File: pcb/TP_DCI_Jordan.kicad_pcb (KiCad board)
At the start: 2 copper layers, 50.6 x 30 mm, 19 parts, among them J1 MICRO, J2 Display, SW1 SW_DIP_x03, U1 PCF8574

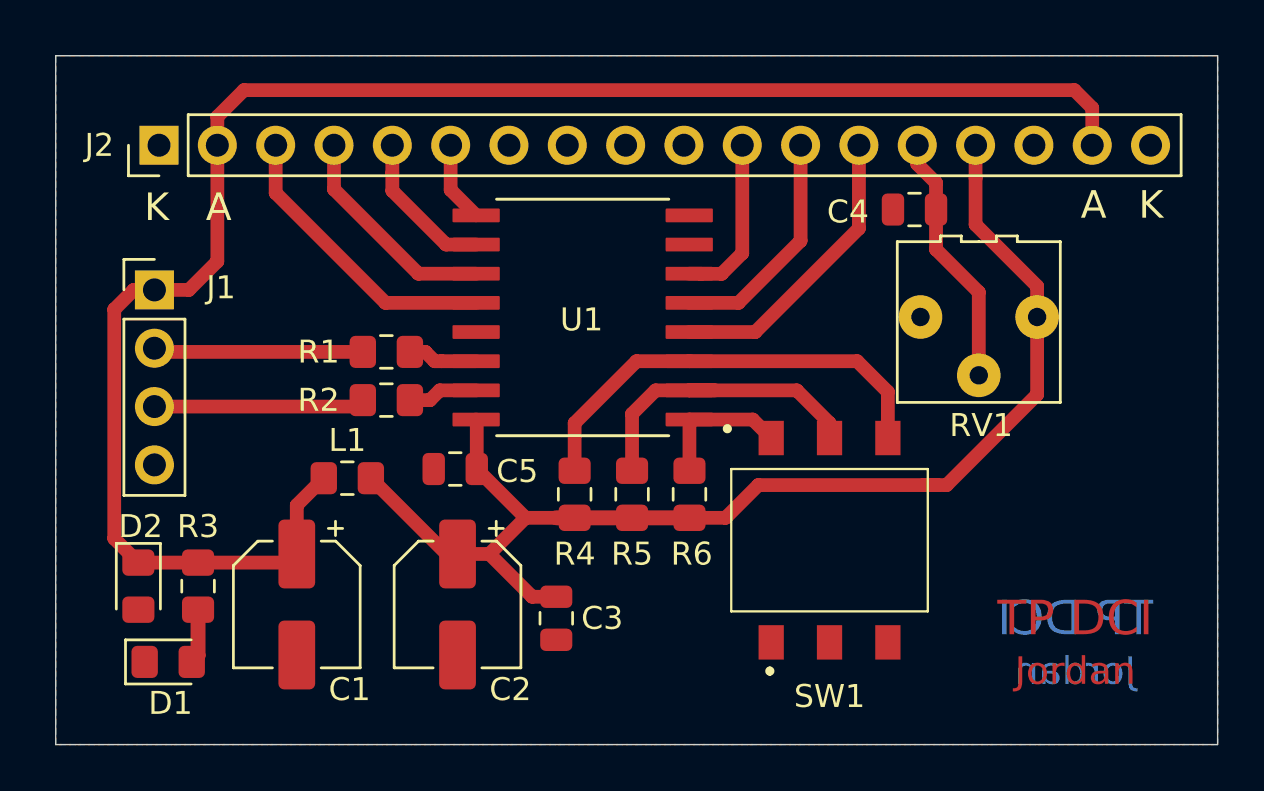
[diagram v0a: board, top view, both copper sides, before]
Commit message: medición longitudes de PCB
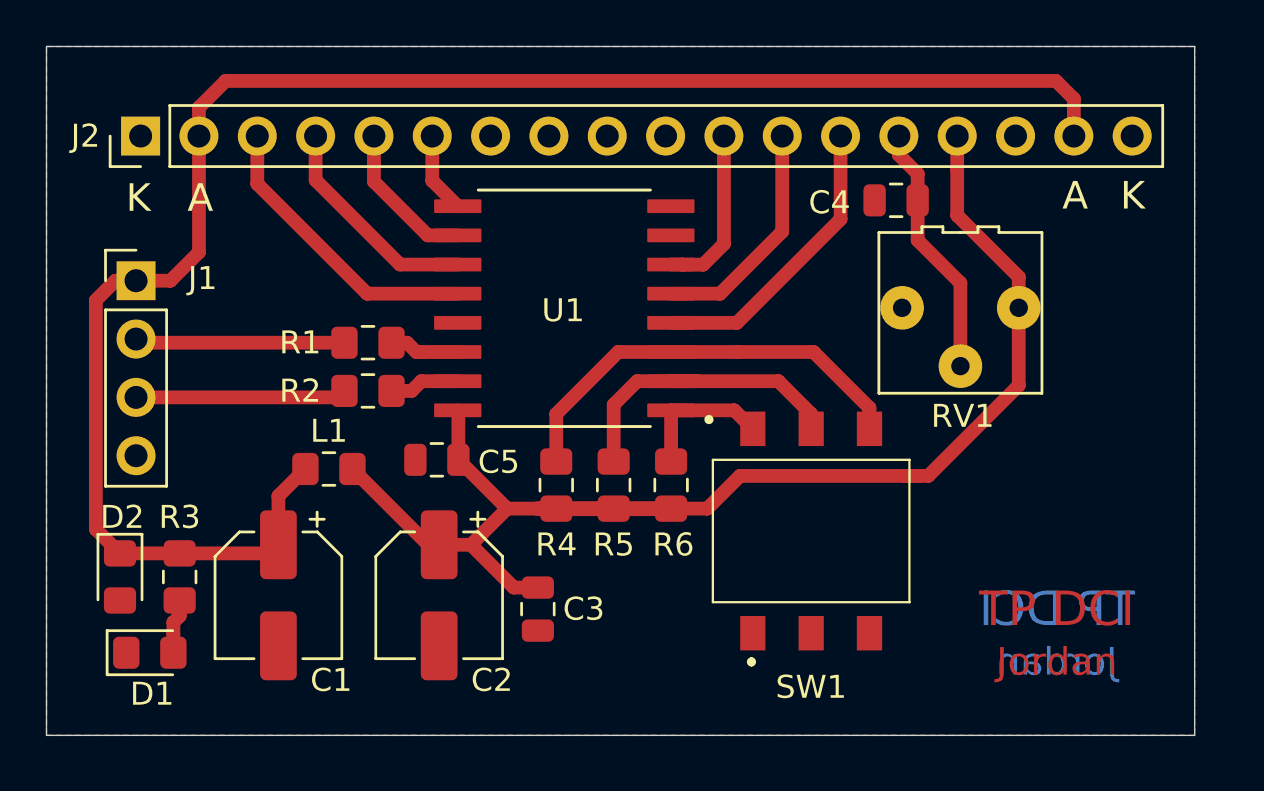
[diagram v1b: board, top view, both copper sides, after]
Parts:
- moved C1 0.89 mm to (91.1, 133.9)
- moved C2 0.89 mm to (98.1, 133.9)
- moved J2 0.89 mm to (85.1, 113.9)
- moved C3 0.89 mm to (102.4, 134.5)
- moved C5 0.89 mm to (98.0, 128.0)
- moved D1 0.89 mm to (85.5, 136.4)
- moved D2 0.89 mm to (84.2, 133.1)
- moved L1 0.89 mm to (93.3, 128.4)
- moved R2 0.89 mm to (95.0, 125.0)
- moved R3 0.89 mm to (86.8, 133.1)
- moved R4 0.89 mm to (103.2, 129.1)
- moved R5 0.89 mm to (105.7, 129.1)
- moved R6 0.89 mm to (108.2, 129.1)
- moved RV1 0.89 mm to (120.8, 121.6)
- moved SW1 0.89 mm to (114.3, 131.1)
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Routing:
- net Net-(R4-Pad1): track 19.4 -> 18.7 mm
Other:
- board size 50.6 x 30 mm -> 50 x 30 mm
